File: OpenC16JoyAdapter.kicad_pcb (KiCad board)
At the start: 2 copper layers, 31 x 50.5 mm, 16 parts, among them J1 DB9_MALE, J2 TO_C16_MINI_DIN_8, Q1 BC548, Q2 BC547, Q3 BC547, SW1 SW_PIN5_POWER, SW2 SW_LIGHTPEN, U1 74LS244

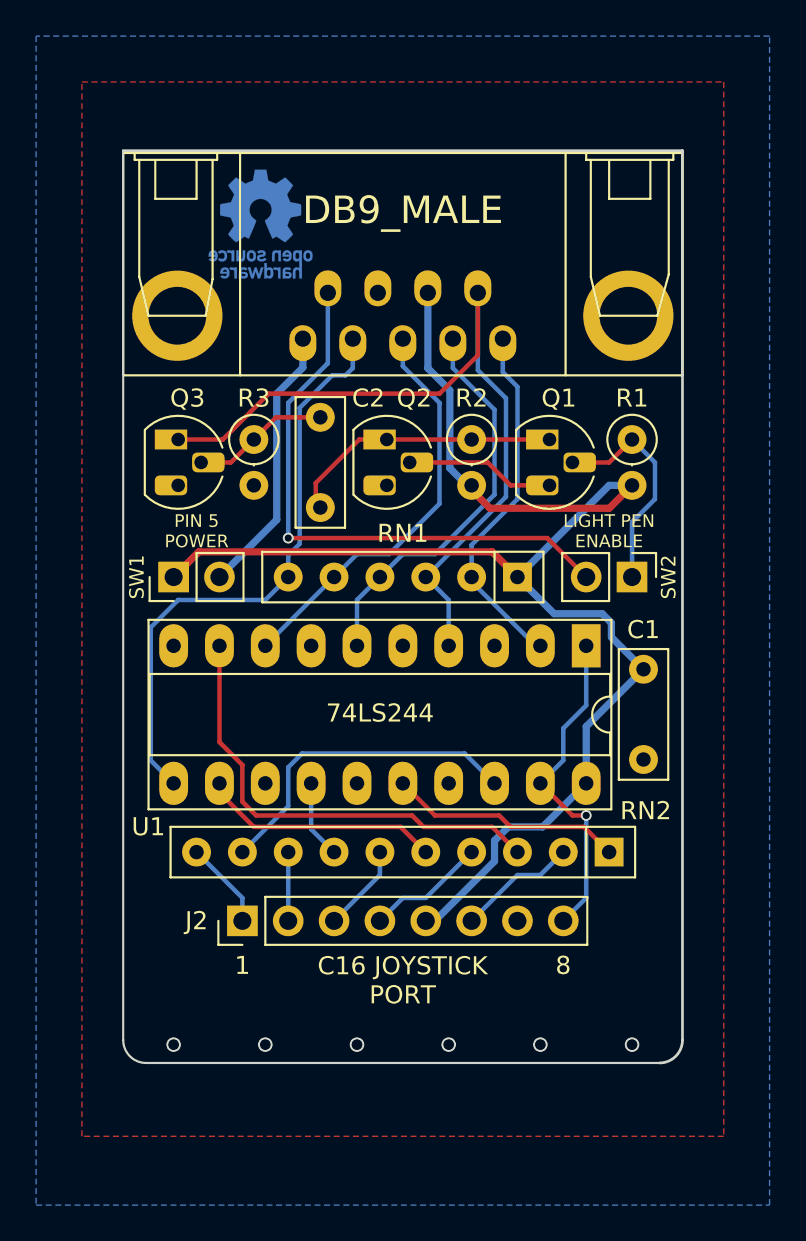
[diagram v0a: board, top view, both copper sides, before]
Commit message: Final touches
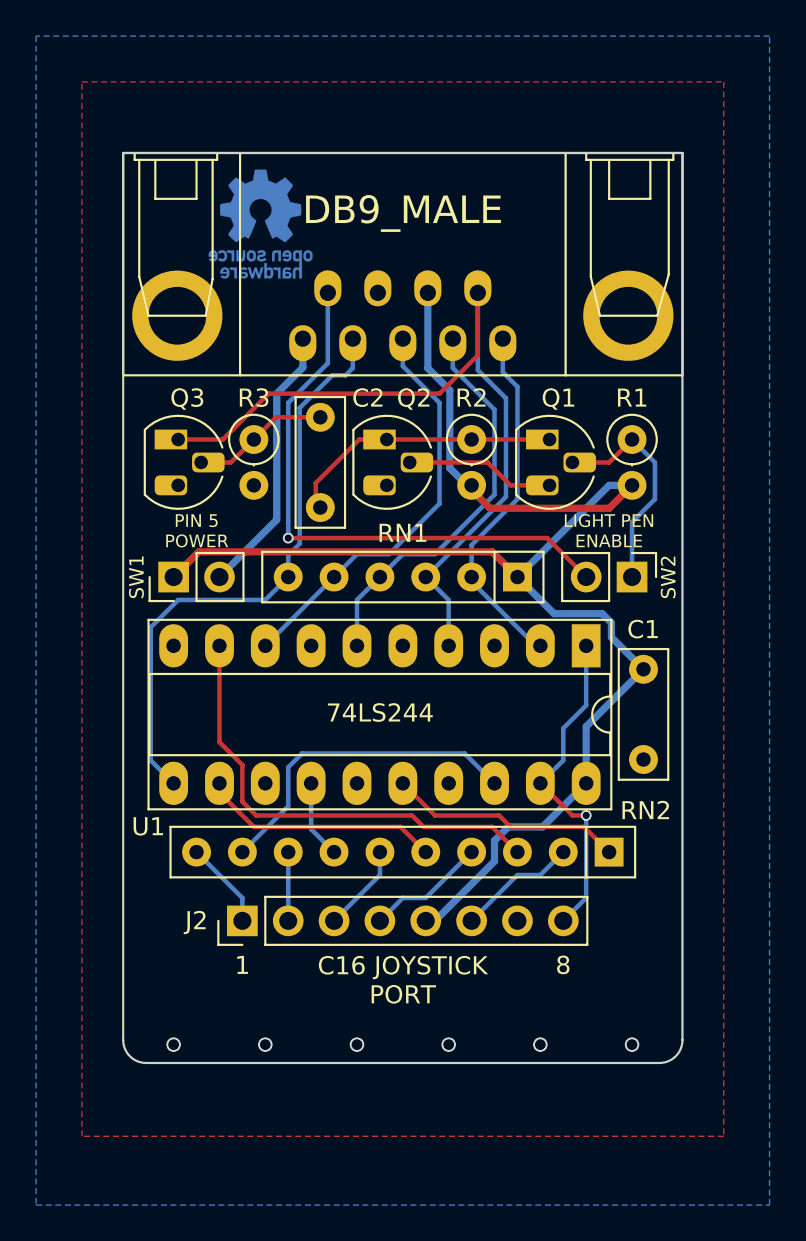
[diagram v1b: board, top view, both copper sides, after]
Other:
- board size 31 x 50.5 mm -> 31 x 50.4 mm
